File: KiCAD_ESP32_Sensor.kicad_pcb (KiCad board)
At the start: 2 copper layers, 50 x 40 mm, 24 parts, among them J1 USB_C_Receptacle_USB2.0_16P, J2 VL53L0X_Module, Q1 MMBT3904, Q2 MMBT3904, U1 CH340C, U2 AMS1117-3.3, U3 ESP32-WROOM-32E

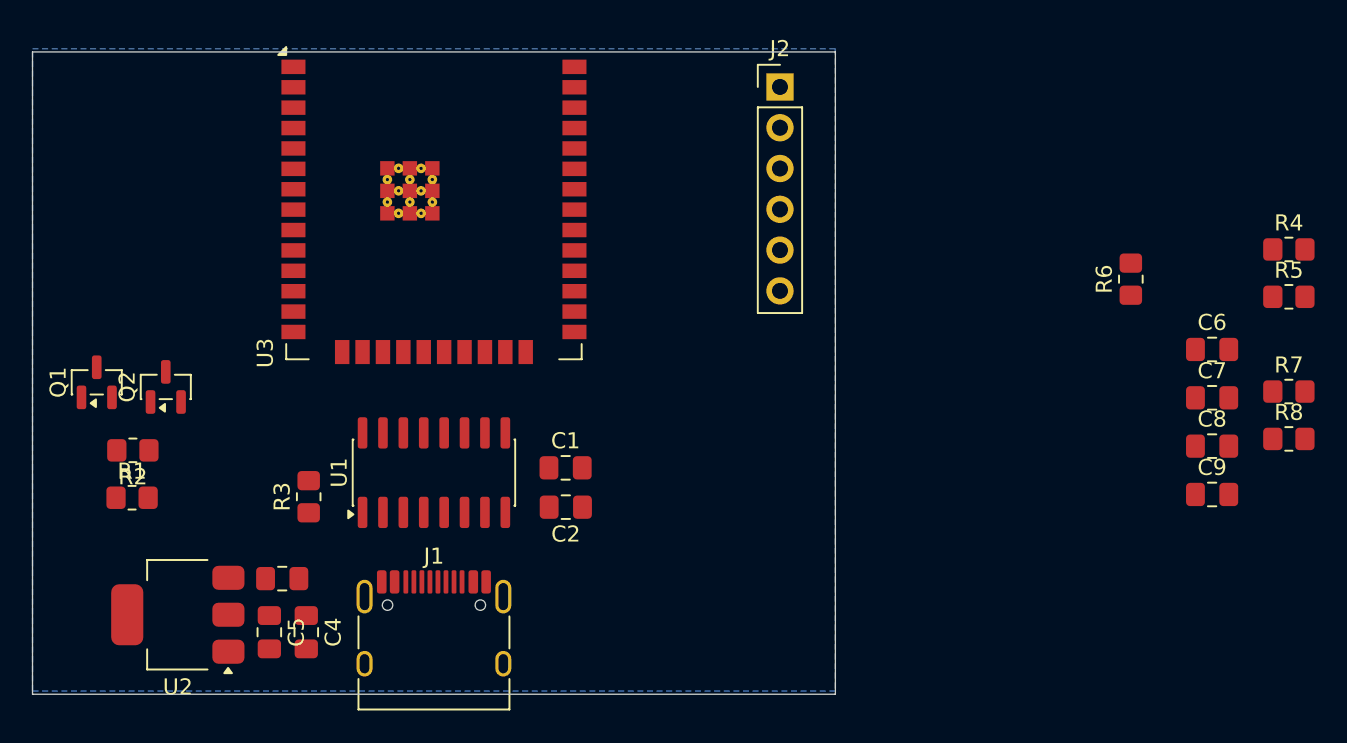
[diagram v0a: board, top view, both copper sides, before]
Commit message: Finished rough PCB design, will finalize later
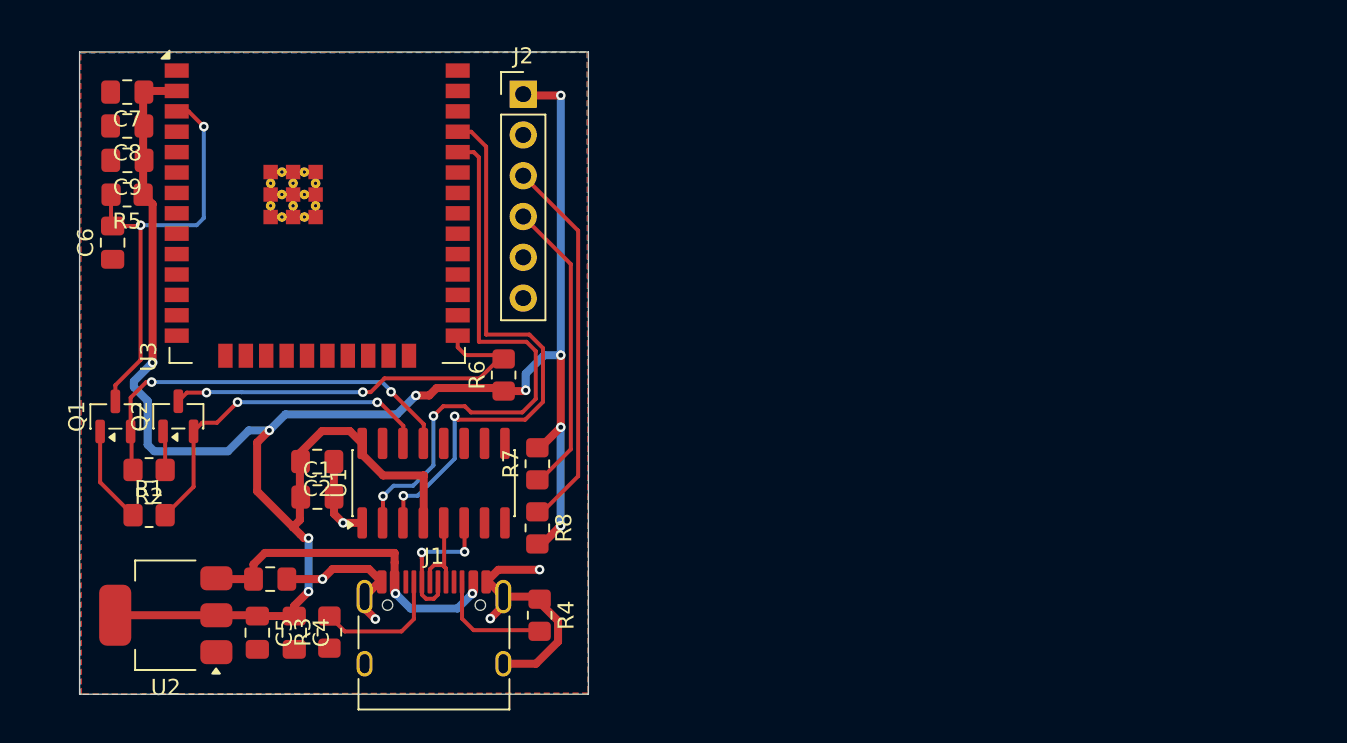
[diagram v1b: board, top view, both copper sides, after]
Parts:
- moved R5 72.6 mm to (55.9, 59.1), turned to 180 degrees
- moved C9 70.7 mm to (55.9, 57.0), turned to 180 degrees
- moved C8 70.4 mm to (55.9, 54.8), turned to 180 degrees
- moved C7 70.2 mm to (55.9, 52.7), turned to 180 degrees
- moved C6 68.8 mm to (55.0, 62.1), turned to 90 degrees
- moved R4 51.9 mm to (81.6, 85.3), turned to -90 degrees
- moved R8 47.1 mm to (81.4, 79.8), turned to -90 degrees
- moved R7 47.0 mm to (81.4, 75.8), turned to 90 degrees
- moved R6 39.5 mm to (79.3, 70.3)
- moved J2 16.0 mm to (80.6, 52.8)
- moved C2 15.7 mm to (67.7, 75.7)
- moved C1 15.6 mm to (67.7, 77.9)
- moved R3 8.53 mm to (68.5, 86.3)
- moved U3 7.27 mm to (67.7, 56.6)
- moved Q1 2.42 mm to (55.2, 72.9)
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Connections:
- C7 pad 2: Net-(C7-Pad2) -> GND
- C9 pad 2: Net-(C7-Pad2) -> GND
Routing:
- net +3.3V: track 0.14 -> 130.0 mm, vias 0 -> 10
- net RXD: track 0.00 -> 35.0 mm, vias 0 -> 2
- net TXD: track 0.00 -> 34.9 mm, vias 0 -> 2
- net GND: track 0.00 -> 31.0 mm, vias 0 -> 5
- net EN: track 0.00 -> 27.3 mm, vias 0 -> 2
- net DTR: track 0.00 -> 24.9 mm, vias 0 -> 2
- net IO0: track 0.00 -> 24.8 mm, vias 0 -> 2
- net SCL: track 0.00 -> 23.4 mm
- net +5V: track 0.00 -> 21.2 mm, vias 0 -> 2
- net RTS: track 0.00 -> 20.8 mm, vias 0 -> 2
- net SDA: track 0.00 -> 18.4 mm
- net USB_D_MINUS: track 0.00 -> 9.78 mm, vias 0 -> 2
- net Net-(J1-CC1): track 0.00 -> 8.29 mm
- net Net-(J1-CC2): track 0.00 -> 6.96 mm
- net USB_D_PLUS: track 0.00 -> 6.33 mm
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- added copper zone on F.Cu, net GND
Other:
- board size 50 x 40 mm -> 31.7 x 40 mm
